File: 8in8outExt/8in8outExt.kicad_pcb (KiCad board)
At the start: 2 copper layers, 49 parts, among them P1 CONN_10X2, SW1 SPST, SW2 SPST, SW3 SPST, SW4 SPST, SW5 SPST, SW6 SPST, SW7 SPST, SW8 SPST, U1 ULN2803, U2 ULN2803

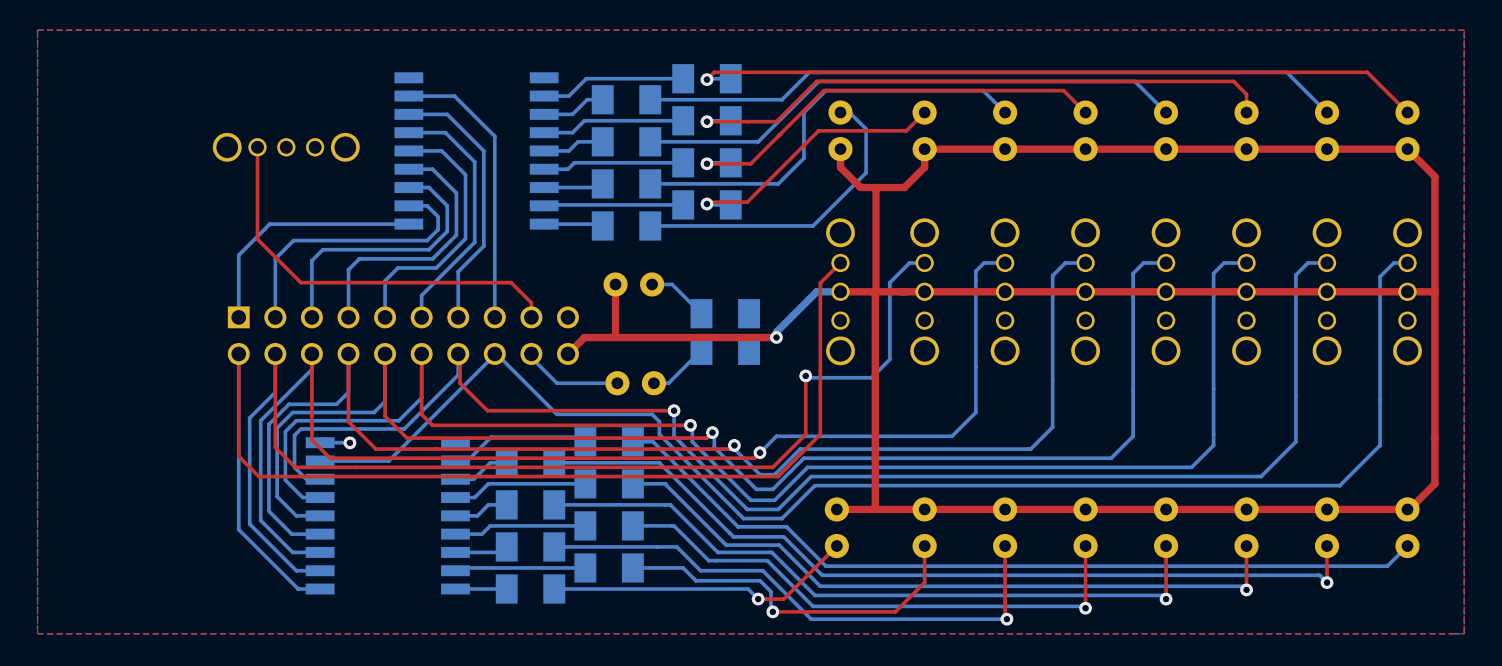
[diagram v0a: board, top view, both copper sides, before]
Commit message: Final pour prod
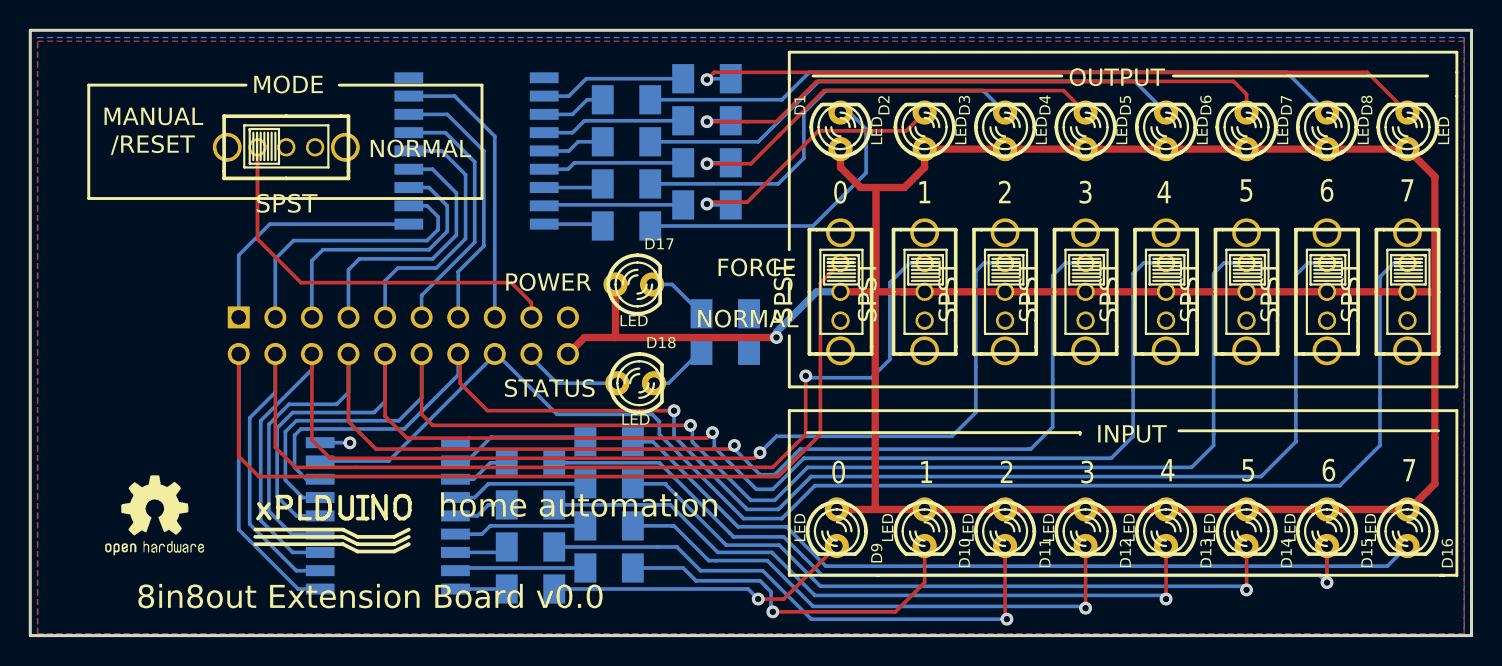
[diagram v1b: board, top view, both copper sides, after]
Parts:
- added G***: LOGO, OSHWLOGO0.3IN, F.Cu at (91.2, 103.9)
- moved logo_xplduino 9.70 mm to (107.3, 108.8)
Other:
- board outline added: 100.1 x 42 mm
- board text added: "8in8out Extension Board v0.0"
- board text added: "MANUAL /RESET"
- board text added: "MODE"
- board text removed: "RESET"
